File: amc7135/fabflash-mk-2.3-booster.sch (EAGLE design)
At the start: 23 parts, among them Q1 MOSFET-PCHANNELIRLML2244, U1 LM2735Y

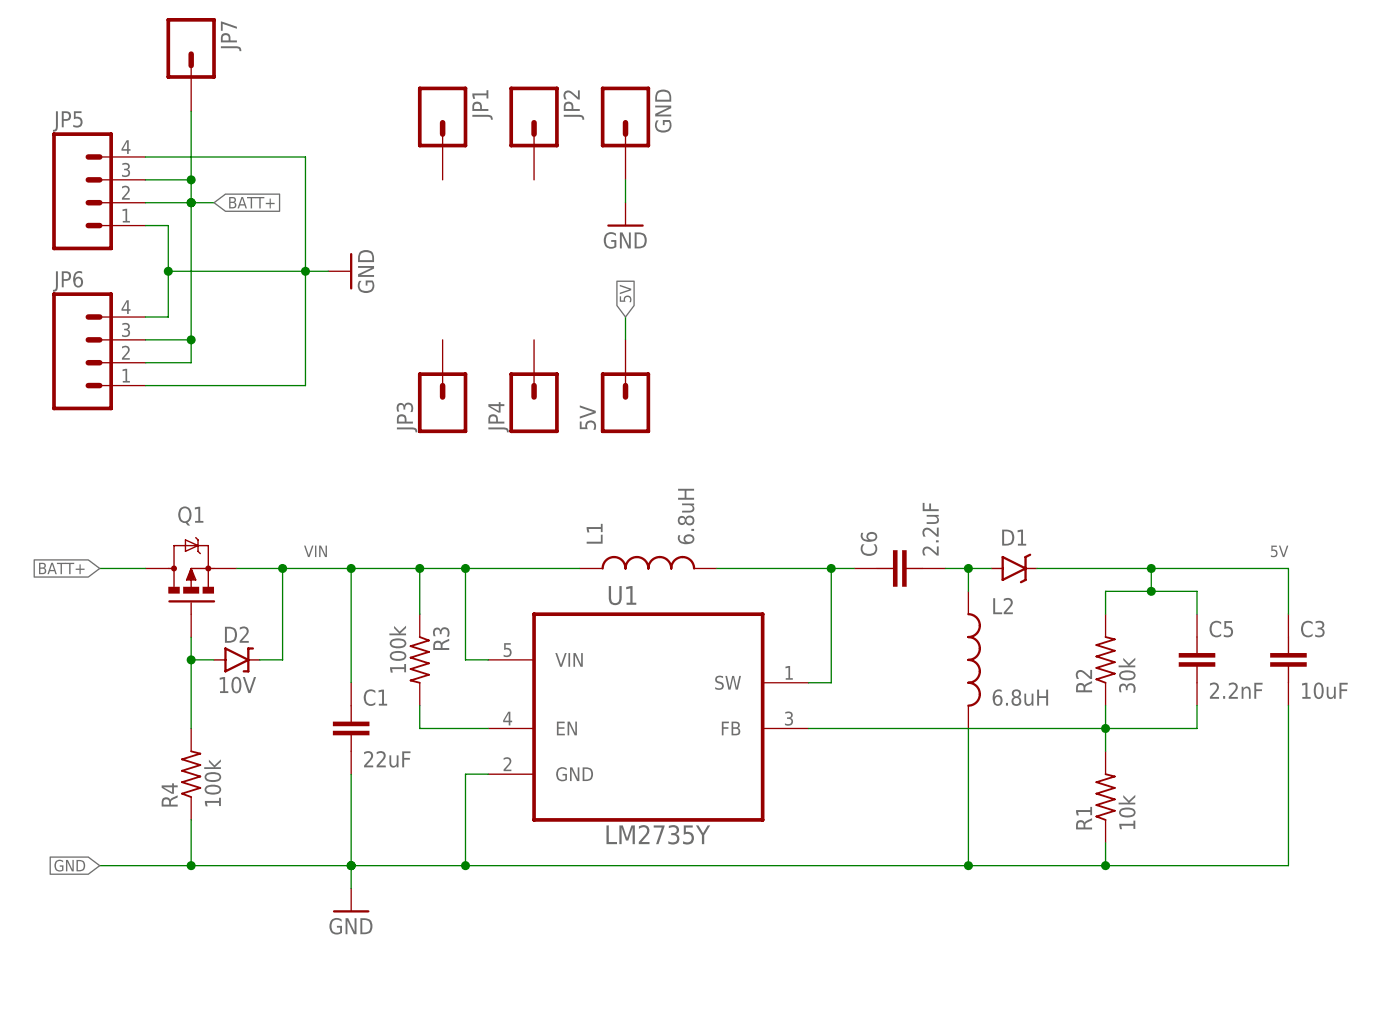
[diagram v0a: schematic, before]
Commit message: finishing touches hopefully
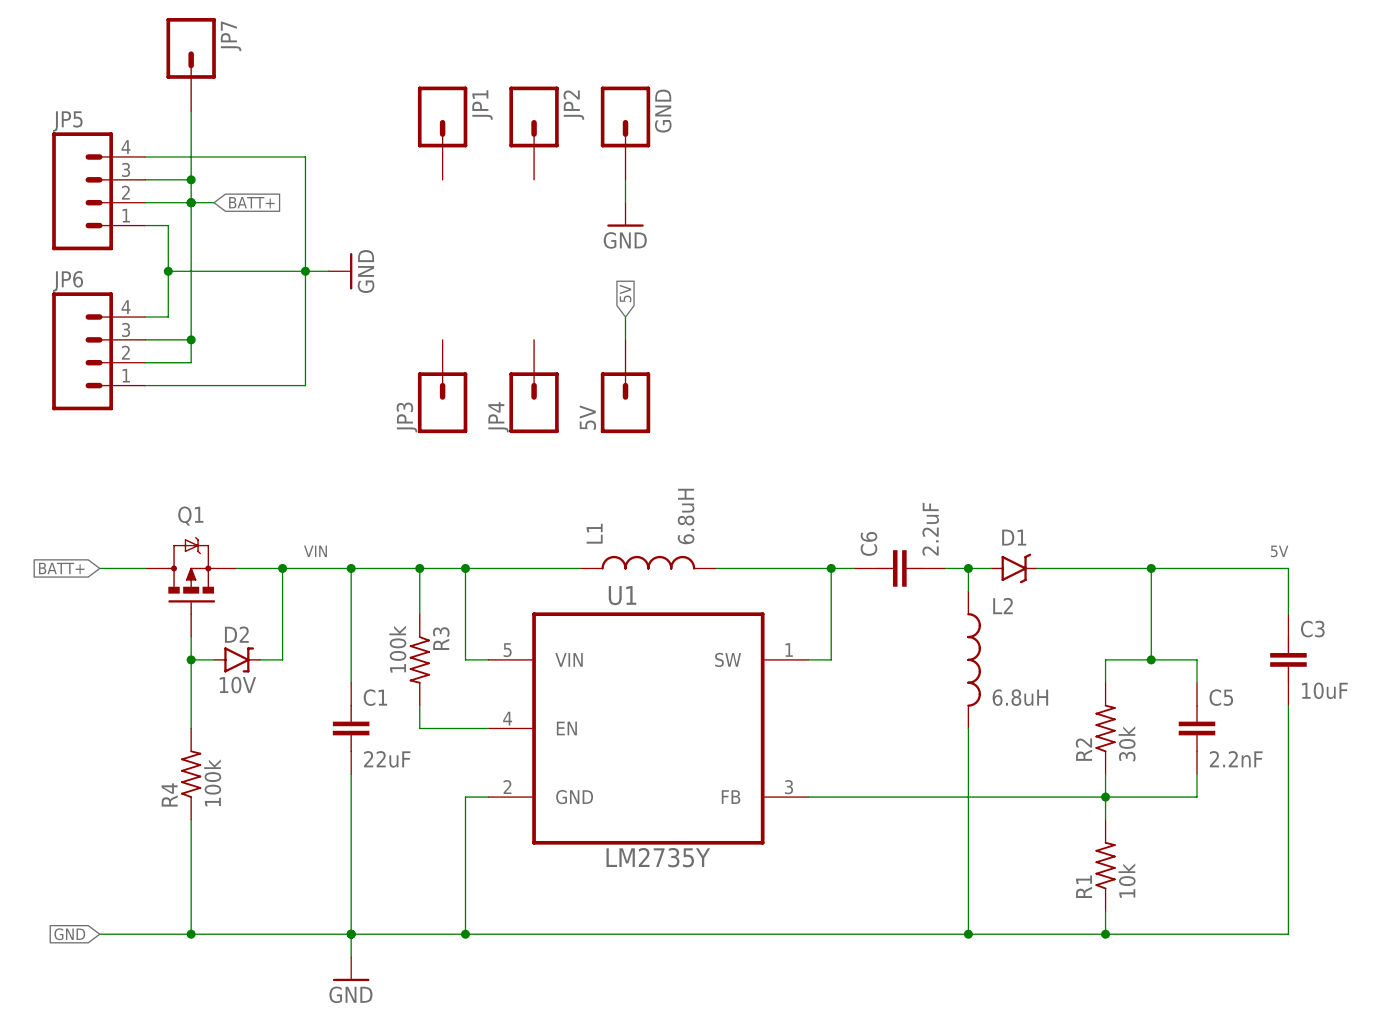
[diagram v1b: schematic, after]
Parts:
- D1: device A_butts:DIODE-SCHOTTKYB340A -> A_butts:DIODE-SCHOTTKYSMA
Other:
- moved on the sheet: C5, R1, R2, U1
